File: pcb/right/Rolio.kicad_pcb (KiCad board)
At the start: 2 copper layers, 141.8 x 83.9 mm, 110 parts, among them Q1 AO3400A, SW4 SW_DIP_x01

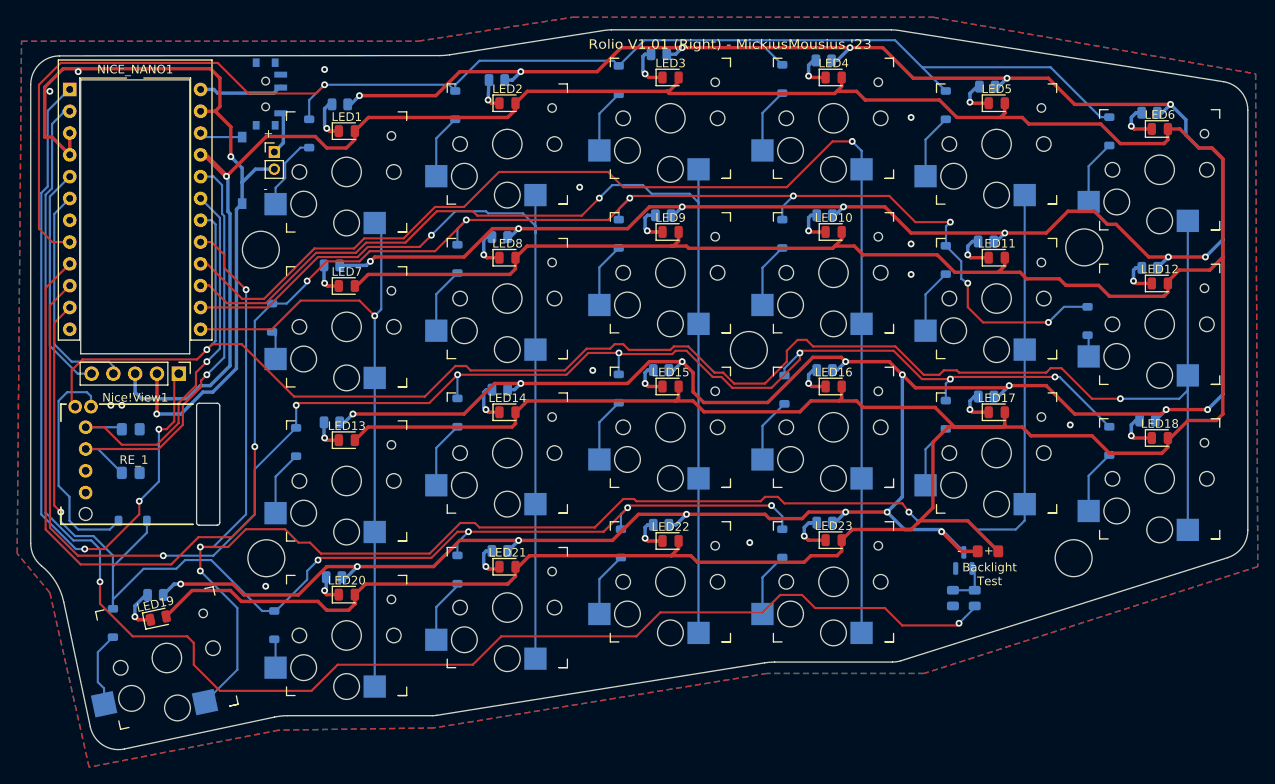
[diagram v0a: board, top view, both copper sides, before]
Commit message: Check in V1.0
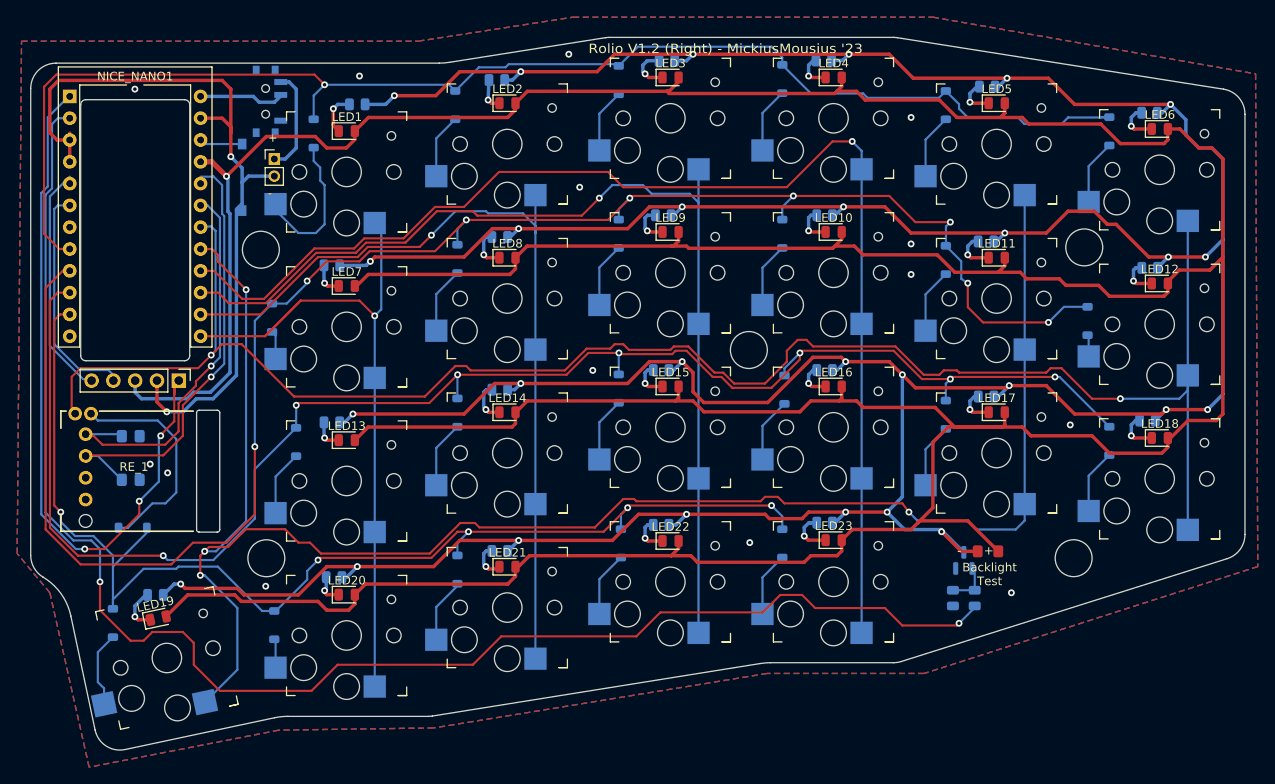
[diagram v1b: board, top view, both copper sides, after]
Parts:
- H2: moved to B.Cu
- moved R3 2.03 mm to (85.3, 41.9)
- moved R5 1.20 mm to (121.4, 36.8)
- moved SW4 0.86 mm to (75.0, 41.6)
- moved BATT1 0.81 mm to (75.7, 48.3)
- moved C1 0.81 mm to (59.0, 80.6)
- moved C2 0.81 mm to (58.9, 85.6)
- moved Nice!View1 0.81 mm to (64.5, 74.1)
- moved RE_1 0.81 mm to (59.3, 84.1)
- moved NICE_NANO1 0.81 mm to (51.8, 41.0)
- moved RESET1 0.81 mm to (71.9, 50.4)
- moved D19 0.81 mm to (59.2, 91.2)
- moved D1 0.53 mm to (80.3, 45.3)
- turned H2 to 180 degrees
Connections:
- SW4 pad 1: Net-(BATT1-+) -> (no net)
- SW4 pad 3: (no net) -> Net-(BATT1-+)
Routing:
- net row0: track 168.9 -> 160.2 mm
- net Net-(D1-A): track 8.79 -> 16.7 mm
- net Net-(BATT1-+): track 4.80 -> 12.1 mm
- net col5: track 76.0 -> 82.2 mm
- net BL_GND: track 523.9 -> 521.1 mm
- net GND: track 91.8 -> 89.0 mm, vias 15 -> 16
- net row3: track 143.6 -> 141.5 mm
- net col1: track 204.5 -> 203.6 mm
- net Net-(D19-A): track 26.7 -> 25.8 mm
- net BL_CTRL: track 177.4 -> 178.2 mm
- net row2: track 187.8 -> 188.5 mm
- net col0: track 204.5 -> 203.8 mm
- net VCC: track 562.6 -> 562.0 mm
- net CS: track 83.7 -> 84.2 mm
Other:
- board size 141.8 x 83.9 mm -> 141.5 x 83 mm
- board text added: "+"
- board text added: "Rolio V1.2 (Right) - MickiusMousius '23"
- board text removed: "Rolio V1.01 (Right) - MickiusMousius '23"
